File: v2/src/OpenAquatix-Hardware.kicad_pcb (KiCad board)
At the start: 4 copper layers, 96.2 x 96.2 mm, 279 parts, among them J1 USB_B_Micro, J2 Conn_ARM_JTAG_SWD_10, J3 Screw_Terminal_01x02, J4 Screw_Terminal_01x03, Q1 CSD19534Q5A, Q2 BSS138, SW1 SW_Push, SW2 SW_Push, SW3 CJS-1200TA, U1 STM32H723VETx, U10 TPD4E05U06DQA, U11 SSF2215, U12 TPS72301DBV, U13 LM5155DSSR, U14 TLV9061xDBV, U15 OPA333xxD, U16 TLV9061xDBV, U17 PGA113, U18 TPA3132D2RHBR, U19 TLV9151xDBV, U2 TLV75733PDYDR, U20 TLV9151xDBV, U21 SN74LVC1G14DBV, U22 TLP241BTP1_F, U23 TLP241BTP1_F, U24 TLV9061xDBV, U25 TLV9061xDBV, U3 TLV75733PDYDR, U4 TPSM84209RKHR, U5 TPD4E05U06DQA, U6 TPD4E05U06DQA, U7 INA219AIDCNR, U8 SN74LXC1T14DCKR, U9 TPS60403DBV, Y1 8 MHz

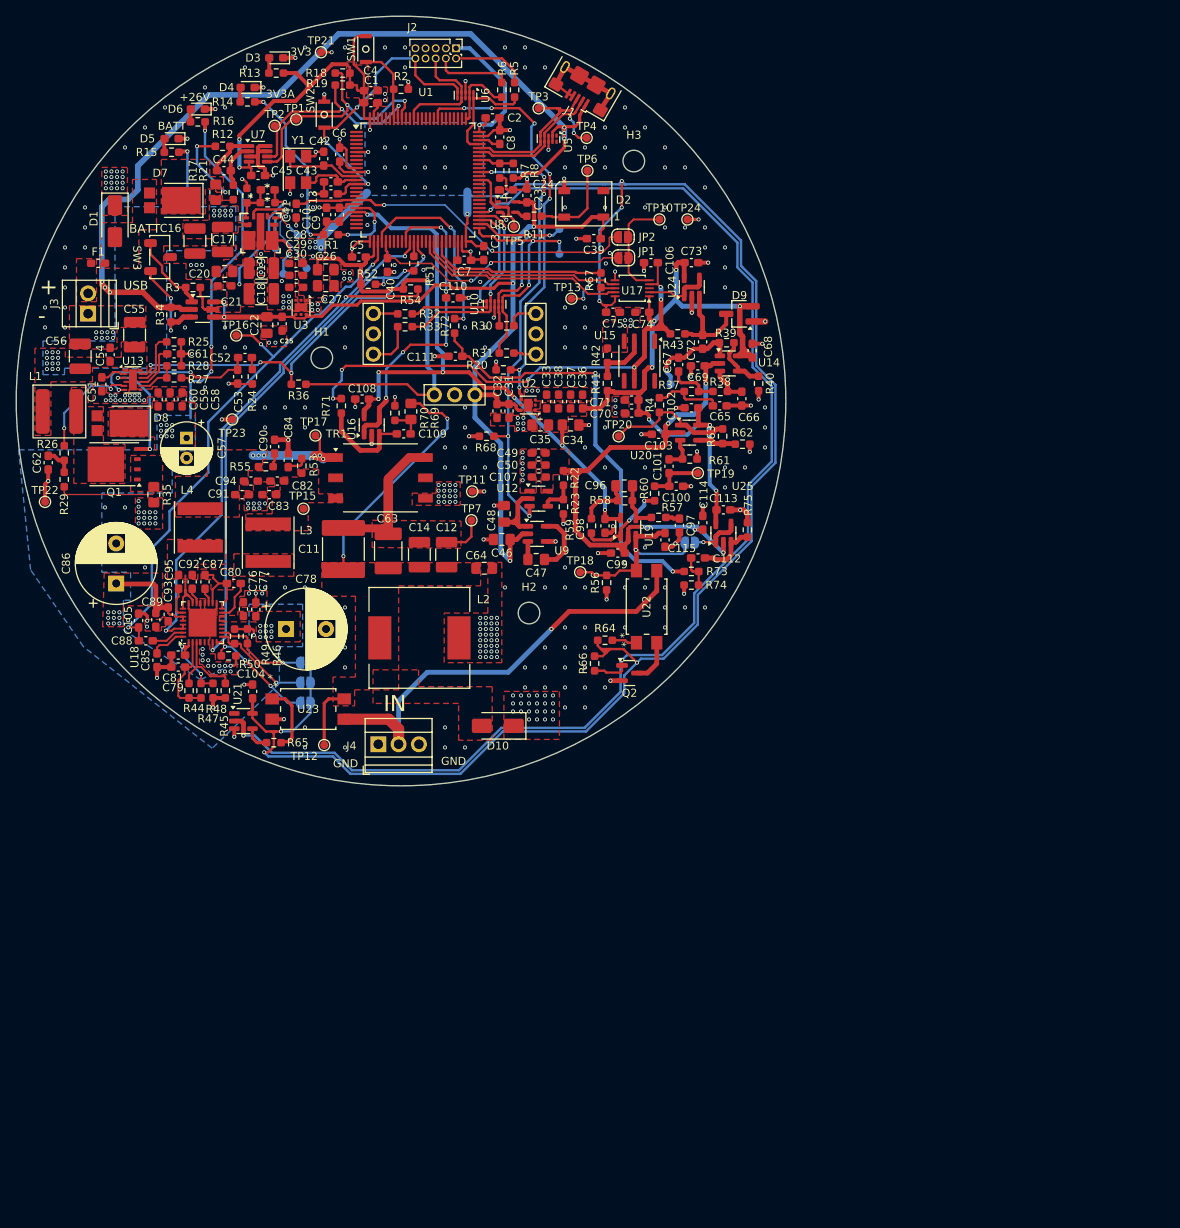
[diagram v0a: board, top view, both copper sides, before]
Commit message: v2.0 final version including minor hardware revisions
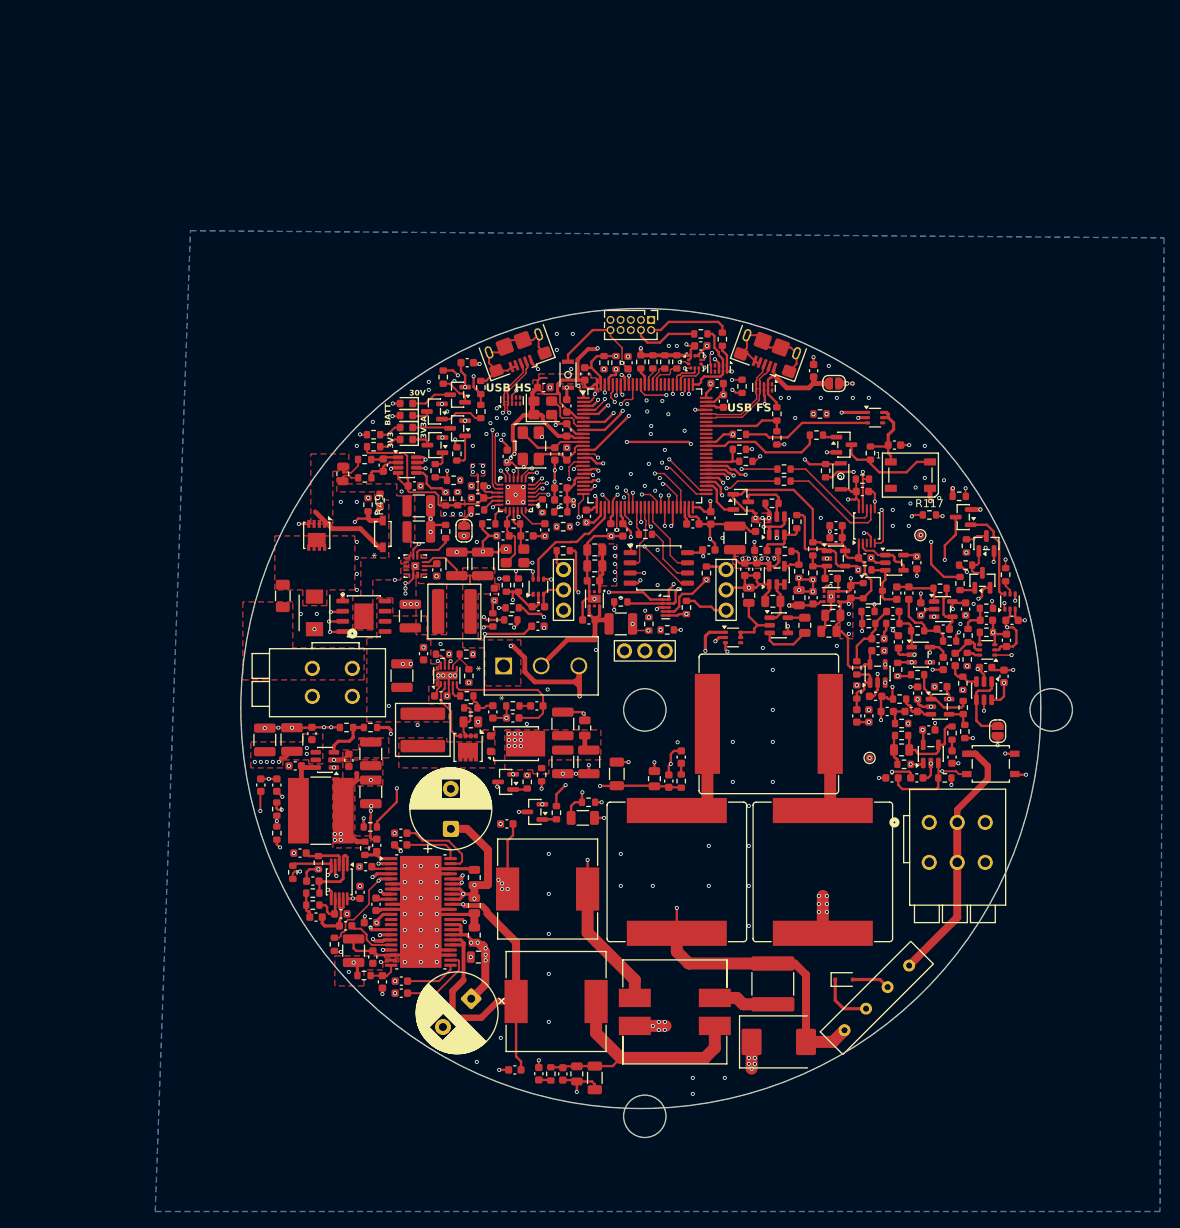
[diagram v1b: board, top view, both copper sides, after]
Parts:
- removed JP4, JP5: SolderJumper_2_Open, Jumper:SolderJumper-2_P1.3mm_Open_RoundedPad1.0x1.5mm
- removed JP6: ~, Jumper:SolderJumper-2_P1.3mm_Open_RoundedPad1.0x1.5mm
- removed TP10, TP14, TP3, TP4, TP5, TP6, TP8, TP9: TestPoint_Small, TestPoint:TestPoint_Pad_D1.0mm
- removed TP11, TP12, TP13, TP15, TP16, TP17, TP18, TP19, TP20, TP21, TP22, TP23, TP24, TP7: TestPoint, TestPoint:TestPoint_Pad_D1.0mm
- removed TP25, TP26, TP27, TP28: ~, TestPoint:TestPoint_Pad_D1.0mm
- removed TR1: Wuerth_760390012, Transformer_SMD:Transformer_Wuerth_750315371
- added C116: 100n, Capacitor_SMD:C_0603_1608Metric, F.Cu at (137.0, 97.1)
- added C117: 100n, Capacitor_SMD:C_0603_1608Metric, F.Cu at (134.1, 97.9)
- added C118: ~, Capacitor_SMD:C_0603_1608Metric, F.Cu at (130.9, 108.5)
- added C119: 33n, Capacitor_SMD:C_0603_1608Metric, F.Cu at (138.4, 105.9)
- added C120: 10u, Capacitor_SMD:C_0805_2012Metric, F.Cu at (132.1, 105.0)
- added C121: 10n, Capacitor_SMD:C_0603_1608Metric, F.Cu at (130.3, 100.2)
- added C122: 2u2, Capacitor_SMD:C_0603_1608Metric, F.Cu at (133.3, 100.2)
- added C123: 68n,200V,5%,C0G/NP0, Capacitor_SMD:C_2220_5750Metric, F.Cu at (116.0, 134.2)
- added C128: 100n, Capacitor_SMD:C_0603_1608Metric, F.Cu at (129.2, 92.6)
- added C129: 100n, Capacitor_SMD:C_0603_1608Metric, F.Cu at (128.8, 98.3)
- added C130: 100n, Capacitor_SMD:C_0603_1608Metric, F.Cu at (137.3, 94.2)
- added C131: 100n, Capacitor_SMD:C_0603_1608Metric, F.Cu at (131.7, 91.5)
- added C132: 1n, Capacitor_SMD:C_0603_1608Metric, F.Cu at (128.0, 100.8)
- added C133: 100n, Capacitor_SMD:C_0603_1608Metric, F.Cu at (140.1, 87.4)
- added C134: 100n, Capacitor_SMD:C_0603_1608Metric, F.Cu at (134.5, 87.4)
- added C135: 1n, Capacitor_SMD:C_0603_1608Metric, F.Cu at (126.5, 100.8)
- added C136: 1n, Capacitor_SMD:C_0603_1608Metric, F.Cu at (129.2, 91.1)
- added C137: 1n, Capacitor_SMD:C_0603_1608Metric, F.Cu at (131.0, 87.7)
- added C138: 1n, Capacitor_SMD:C_0603_1608Metric, F.Cu at (137.3, 89.9)
- added C139: 1n, Capacitor_SMD:C_0603_1608Metric, F.Cu at (133.0, 85.4)
- added C140: 100n, Capacitor_SMD:C_0603_1608Metric, F.Cu at (123.3, 83.6)
- added C141: 100n, Capacitor_SMD:C_0603_1608Metric, F.Cu at (123.9, 78.5)
- added C142: 1u, Capacitor_SMD:C_0603_1608Metric, F.Cu at (123.9, 77.0)
- added C143: 100n, Capacitor_SMD:C_0603_1608Metric, F.Cu at (131.5, 85.4)
- added C144: 100n, Capacitor_SMD:C_0603_1608Metric, F.Cu at (134.0, 81.6)
- added C145: 100n, Capacitor_SMD:C_0603_1608Metric, F.Cu at (127.5, 81.0)
- added C146: 100n, Capacitor_SMD:C_0603_1608Metric, F.Cu at (127.2, 72.7)
- added C147: 100n, Capacitor_SMD:C_0603_1608Metric, F.Cu at (145.9, 88.8)
- added D11: BAT54WS, Diode_SMD:D_SOD-323F, F.Cu at (124.9, 133.7)
- added G***: LOGO, OpenAquatix-Hardware_footprints:OpenAquatix_logo, B.Cu at (100.0, 90.0)
- added J6: 2601-1103, OpenAquatix-Hardware_footprints:CONN3_2601-1103_WAG, F.Cu at (135.6, 114.1)
- added K1: 3570.1419.051, OpenAquatix-Hardware_footprints:3570.1419.xxx, F.Cu at (129.0, 136.0)
- added L5: 33u, OpenAquatix-Hardware_footprints:CDRH127L125NP, F.Cu at (87.8, 122.4)
- added L6: 136u, OpenAquatix-Hardware_footprints:B82477D4xxxM900, F.Cu at (103.8, 137.8)
- added L7: 100u, Inductor_SMD:L_Pulse_PA4344, F.Cu at (104.0, 120.2)
- added L8: 100u, Inductor_SMD:L_Pulse_PA4344, F.Cu at (115.5, 101.8)
- added L9: 100u, Inductor_SMD:L_Pulse_PA4344, F.Cu at (122.2, 120.2)
- added Q10: BSS138, Package_TO_SOT_SMD:SOT-23, F.Cu at (112.0, 74.0)
- added Q11: DMP3068L-7, Package_TO_SOT_SMD:SOT-23, F.Cu at (142.7, 79.2)
- added Q12: BSS138, Package_TO_SOT_SMD:SOT-23, F.Cu at (142.2, 83.8)
- added Q13: BSS138, Package_TO_SOT_SMD:SOT-23, F.Cu at (139.8, 75.9)
- added Q3: Si7617DN, Package_SO:Vishay_PowerPAK_1212-8_Single, F.Cu at (59.0, 78.2)
- added Q4: BSS138, Package_TO_SOT_SMD:SOT-23, F.Cu at (82.6, 109.0)
- added Q5: BSS138, Package_TO_SOT_SMD:SOT-23, F.Cu at (86.2, 112.8)
- added Q6: BSS138, Package_TO_SOT_SMD:SOT-23, F.Cu at (73.8, 66.9)
- added Q7: BSS138, Package_TO_SOT_SMD:SOT-23, F.Cu at (76.6, 64.8)
- added Q8: BSS138, Package_TO_SOT_SMD:SOT-23, F.Cu at (73.7, 62.7)
- added Q9: BSS138, Package_TO_SOT_SMD:SOT-23, F.Cu at (76.6, 60.6)
- added R100: 56k, Resistor_SMD:R_0603_1608Metric, F.Cu at (139.8, 99.7)
- added R101: 8k66, Resistor_SMD:R_0603_1608Metric, F.Cu at (134.1, 95.6)
- added R102: 2k05, Resistor_SMD:R_0603_1608Metric, F.Cu at (131.6, 95.0)
- added R103: 16k9, Resistor_SMD:R_0603_1608Metric, F.Cu at (126.5, 97.8)
- added R104: 10k, Resistor_SMD:R_0603_1608Metric, F.Cu at (126.5, 94.8)
- added R105: 1k91, Resistor_SMD:R_0603_1608Metric, F.Cu at (128.0, 89.2)
- added R106: 28k, Resistor_SMD:R_0603_1608Metric, F.Cu at (131.0, 89.2)
- added R107: 6k19, Resistor_SMD:R_0603_1608Metric, F.Cu at (134.1, 90.1)
- added R108: 1k18, Resistor_SMD:R_0603_1608Metric, F.Cu at (138.1, 91.4)
- added R109: 17k4, Resistor_SMD:R_0603_1608Metric, F.Cu at (136.9, 84.8)
- added R110: 10k, Resistor_SMD:R_0603_1608Metric, F.Cu at (121.0, 79.9)
- added R111: 10k, Resistor_SMD:R_0603_1608Metric, F.Cu at (121.0, 82.9)
- added R112: 10k, Resistor_SMD:R_0603_1608Metric, F.Cu at (127.5, 82.5)
- added R113: 100k, Resistor_SMD:R_0603_1608Metric, F.Cu at (139.3, 73.3)
- added R114: 390R, Resistor_SMD:R_0603_1608Metric, F.Cu at (145.1, 83.1)
- added R115: 100k, Resistor_SMD:R_0603_1608Metric, F.Cu at (127.2, 71.2)
- added R116: 100k, Resistor_SMD:R_0603_1608Metric, F.Cu at (112.2, 59.5)
- added R117: 10k, Resistor_SMD:R_0603_1608Metric, F.Cu at (135.6, 75.6)
- added R76: 100k, Resistor_SMD:R_0603_1608Metric, F.Cu at (79.5, 59.7)
- added R77: 47k, Resistor_SMD:R_0603_1608Metric, F.Cu at (66.9, 73.8)
- added R78: 220R, Resistor_SMD:R_0603_1608Metric, F.Cu at (74.8, 58.4)
- added R79: 100k, Resistor_SMD:R_0603_1608Metric, F.Cu at (96.4, 56.6)
- added R80: 47k, Resistor_SMD:R_0603_1608Metric, F.Cu at (87.1, 108.1)
- added R81: 160k,1%, Resistor_SMD:R_1206_3216Metric, F.Cu at (92.2, 113.5)
- added R82: 1k6,1%, Resistor_SMD:R_0603_1608Metric, F.Cu at (93.0, 111.5)
- added R83: 100k, Resistor_SMD:R_0603_1608Metric, F.Cu at (119.0, 76.5)
- added R84: 2k, Resistor_SMD:R_0603_1608Metric, F.Cu at (115.9, 74.2)
- added R85: 2k49, Resistor_SMD:R_0603_1608Metric, F.Cu at (142.7, 87.3)
- added R86: 732R, Resistor_SMD:R_0603_1608Metric, F.Cu at (140.3, 93.7)
- added R87: 1M, Resistor_SMD:R_0603_1608Metric, F.Cu at (140.4, 90.7)
- added R88: 22R, Resistor_SMD:R_0603_1608Metric, F.Cu at (142.7, 90.3)
- added R89: 100k, Resistor_SMD:R_0603_1608Metric, F.Cu at (139.8, 96.7)
- added R90: 1k, Resistor_SMD:R_0603_1608Metric, F.Cu at (140.2, 79.5)
- added R91: 1k, Resistor_SMD:R_0603_1608Metric, F.Cu at (139.4, 84.2)
- added R92: 100k, Resistor_SMD:R_0603_1608Metric, F.Cu at (140.1, 81.9)
- added R93: 1k, Resistor_SMD:R_0603_1608Metric, F.Cu at (137.5, 108.5)
- added R94: 200R, Resistor_SMD:R_0603_1608Metric, F.Cu at (138.4, 102.9)
- added R95: 91k, Resistor_SMD:R_0603_1608Metric, F.Cu at (132.1, 103.2)
- added R96: 10k, Resistor_SMD:R_0603_1608Metric, F.Cu at (132.4, 106.8)
- added R97: 390R, Resistor_SMD:R_0603_1608Metric, F.Cu at (132.1, 101.7)
- added R98: 86k6, Resistor_SMD:R_0603_1608Metric, F.Cu at (131.8, 98.7)
- added R99: 1k, Resistor_SMD:R_0603_1608Metric, F.Cu at (140.0, 102.7)
- added U26: LM6211, Package_TO_SOT_SMD:SOT-23-5, F.Cu at (135.8, 105.5)
- added U27: LMV641MFX/NOPB, Package_TO_SOT_SMD:SOT-23-5, F.Cu at (136.9, 99.6)
- added U28: LMV641MFX/NOPB, Package_TO_SOT_SMD:SOT-23-5, F.Cu at (129.1, 95.5)
- added U29: LMV641MFX/NOPB, Package_TO_SOT_SMD:SOT-23-5, F.Cu at (134.5, 93.1)
- added U30: LMV641MFX/NOPB, Package_TO_SOT_SMD:SOT-23-5, F.Cu at (137.3, 87.4)
- added U31: LMV641MFX/NOPB, Package_TO_SOT_SMD:SOT-23-5, F.Cu at (123.9, 81.1)
- added U32: LMV641MFX/NOPB, Package_TO_SOT_SMD:SOT-23-5, F.Cu at (131.2, 81.6)
- added U33: PGA113, Package_SO:TSSOP-10_3x3mm_P0.5mm, F.Cu at (127.8, 77.0)
- added U34: TS5A4624, Package_TO_SOT_SMD:SOT-363_SC-70-6, F.Cu at (145.7, 86.5)
- added U35: AQY210S, OpenAquatix-Hardware_footprints:RELAY_AQY_SO4_KS_PAN, F.Cu at (143.2, 106.8)
- added Y2: 8 MHz, Crystal:Crystal_SMD_5032-4Pin_5.0x3.2mm, F.Cu at (85.8, 67.0)
- added Y3: 26 MHz, Crystal:Crystal_SMD_3225-4Pin_3.2x2.5mm, F.Cu at (83.8, 80.8)
- C1, C104, C108, C112, C113, C114, C29, C6, C61, C68, C71, C81, C85, C9: footprint Capacitor_SMD:C_0603_1608Metric_Pad1.08x0.95mm_HandSolder -> Capacitor_SMD:C_0603_1608Metric
- C10, C79: value 1u -> 100n; footprint Capacitor_SMD:C_0603_1608Metric_Pad1.08x0.95mm_HandSolder -> Capacitor_SMD:C_0603_1608Metric
- C100: value 10n -> 1n,50V; footprint Capacitor_SMD:C_0603_1608Metric_Pad1.08x0.95mm_HandSolder -> Capacitor_SMD:C_0603_1608Metric
- C101: value 2u2 -> 1n,50V; footprint Capacitor_SMD:C_0603_1608Metric_Pad1.08x0.95mm_HandSolder -> Capacitor_SMD:C_0603_1608Metric
- C102, C103: value 100n -> 10n,50V; footprint Capacitor_SMD:C_0603_1608Metric_Pad1.08x0.95mm_HandSolder -> Capacitor_SMD:C_0603_1608Metric
- C105: value 1n -> 1u; footprint Capacitor_SMD:C_0603_1608Metric_Pad1.08x0.95mm_HandSolder -> Capacitor_SMD:C_0603_1608Metric
- C106, C65: value C -> 100n; footprint Capacitor_SMD:C_0603_1608Metric_Pad1.08x0.95mm_HandSolder -> Capacitor_SMD:C_0603_1608Metric
- C107, C38: value 1n -> 100n; footprint Capacitor_SMD:C_0603_1608Metric_Pad1.08x0.95mm_HandSolder -> Capacitor_SMD:C_0603_1608Metric
- C109, C69: value 100n -> 1n; footprint Capacitor_SMD:C_0603_1608Metric_Pad1.08x0.95mm_HandSolder -> Capacitor_SMD:C_0603_1608Metric
- C11: value C -> 100n; footprint Capacitor_SMD:C_2220_5750Metric_Pad1.97x5.40mm_HandSolder -> Capacitor_SMD:C_0603_1608Metric
- C110, C40, C41: value 47p -> 100n; footprint Capacitor_SMD:C_0603_1608Metric_Pad1.08x0.95mm_HandSolder -> Capacitor_SMD:C_0603_1608Metric
- C111: value 1n -> 10u; footprint Capacitor_SMD:C_0603_1608Metric_Pad1.08x0.95mm_HandSolder -> Capacitor_SMD:C_0603_1608Metric
- C115: value ~ -> 100n; footprint Capacitor_SMD:C_0603_1608Metric_Pad1.08x0.95mm_HandSolder -> Capacitor_SMD:C_0603_1608Metric
- C12: value C -> 8p; footprint Capacitor_SMD:C_1210_3225Metric_Pad1.33x2.70mm_HandSolder -> Capacitor_SMD:C_0603_1608Metric
- C13: value 100n -> 47p; footprint Capacitor_SMD:C_0603_1608Metric_Pad1.08x0.95mm_HandSolder -> Capacitor_SMD:C_0603_1608Metric
- C14: value C -> 100n; footprint Capacitor_SMD:C_1210_3225Metric_Pad1.33x2.70mm_HandSolder -> Capacitor_SMD:C_0603_1608Metric
- C15: value 330p -> 4u7; footprint Capacitor_SMD:C_0603_1608Metric_Pad1.08x0.95mm_HandSolder -> Capacitor_SMD:C_0603_1608Metric
- C16: value 10u,50V -> 47p; footprint Capacitor_SMD:C_1210_3225Metric_Pad1.33x2.70mm_HandSolder -> Capacitor_SMD:C_0603_1608Metric
- C17: value 10u,50V -> 8p; footprint Capacitor_SMD:C_1210_3225Metric_Pad1.33x2.70mm_HandSolder -> Capacitor_SMD:C_0603_1608Metric
- C18, C19: value 47u -> 100n; footprint Capacitor_SMD:C_1210_3225Metric_Pad1.33x2.70mm_HandSolder -> Capacitor_SMD:C_0603_1608Metric
- C2, C24: value 100n -> 1u; footprint Capacitor_SMD:C_0603_1608Metric_Pad1.08x0.95mm_HandSolder -> Capacitor_SMD:C_0603_1608Metric
- C20: value 10u -> 1u; footprint Capacitor_SMD:C_0805_2012Metric_Pad1.18x1.45mm_HandSolder -> Capacitor_SMD:C_0603_1608Metric
- C21: value 1u -> 10u,50V; footprint Capacitor_SMD:C_0603_1608Metric_Pad1.08x0.95mm_HandSolder -> Capacitor_SMD:C_1210_3225Metric
- C22, C26: value 22u -> 10u,50V; footprint Capacitor_SMD:C_0805_2012Metric_Pad1.18x1.45mm_HandSolder -> Capacitor_SMD:C_1210_3225Metric
- C23: value 100n -> 330n; footprint Capacitor_SMD:C_0603_1608Metric_Pad1.08x0.95mm_HandSolder -> Capacitor_SMD:C_0603_1608Metric
- C25, C31: value 100n -> 2u2; footprint Capacitor_SMD:C_0603_1608Metric_Pad1.08x0.95mm_HandSolder -> Capacitor_SMD:C_0805_2012Metric
- C27: value 22u -> 4u7,50V; footprint Capacitor_SMD:C_0805_2012Metric_Pad1.18x1.45mm_HandSolder -> Capacitor_SMD:C_1210_3225Metric
- C28: value 1u -> 68p; footprint Capacitor_SMD:C_0603_1608Metric_Pad1.08x0.95mm_HandSolder -> Capacitor_SMD:C_0603_1608Metric
- C3, C5: value 100n -> 2u2; footprint Capacitor_SMD:C_0603_1608Metric_Pad1.08x0.95mm_HandSolder -> Capacitor_SMD:C_0603_1608Metric
- C30: value 1n -> 10n; footprint Capacitor_SMD:C_0603_1608Metric_Pad1.08x0.95mm_HandSolder -> Capacitor_SMD:C_0603_1608Metric
- C32: value 10u -> 2u2; footprint Capacitor_SMD:C_0603_1608Metric_Pad1.08x0.95mm_HandSolder -> Capacitor_SMD:C_0805_2012Metric
- C33: value 100p -> 1u; footprint Capacitor_SMD:C_0603_1608Metric_Pad1.08x0.95mm_HandSolder -> Capacitor_SMD:C_0603_1608Metric
- C34: value 22u -> 47u; footprint Capacitor_SMD:C_0805_2012Metric_Pad1.18x1.45mm_HandSolder -> Capacitor_SMD:C_1210_3225Metric
- C35: footprint Capacitor_SMD:C_0805_2012Metric_Pad1.18x1.45mm_HandSolder -> Capacitor_SMD:C_1210_3225Metric
- C36: value 1u -> 1n; footprint Capacitor_SMD:C_0603_1608Metric_Pad1.08x0.95mm_HandSolder -> Capacitor_SMD:C_0603_1608Metric
- C37: value 100n -> 22u; footprint Capacitor_SMD:C_0603_1608Metric_Pad1.08x0.95mm_HandSolder -> Capacitor_SMD:C_1210_3225Metric
- C39: value 100n -> 4u7; footprint Capacitor_SMD:C_0603_1608Metric_Pad1.08x0.95mm_HandSolder -> Capacitor_SMD:C_0603_1608Metric
- C4: value 4u7 -> 100n; footprint Capacitor_SMD:C_0603_1608Metric_Pad1.08x0.95mm_HandSolder -> Capacitor_SMD:C_0603_1608Metric
- C42: value 8p -> 100n; footprint Capacitor_SMD:C_0603_1608Metric_Pad1.08x0.95mm_HandSolder -> Capacitor_SMD:C_0603_1608Metric
- C43: value 8p -> 10u; footprint Capacitor_SMD:C_0603_1608Metric_Pad1.08x0.95mm_HandSolder -> Capacitor_SMD:C_0805_2012Metric
- C44: value 1u -> 22u; footprint Capacitor_SMD:C_0603_1608Metric_Pad1.08x0.95mm_HandSolder -> Capacitor_SMD:C_1210_3225Metric
- C45: value 100n -> 10u,63V; footprint Capacitor_SMD:C_0603_1608Metric_Pad1.08x0.95mm_HandSolder -> Capacitor_SMD:C_1210_3225Metric
- C46, C47: value 2u2 -> 10u,63V; footprint Capacitor_SMD:C_0805_2012Metric_Pad1.18x1.45mm_HandSolder -> Capacitor_SMD:C_1210_3225Metric
- C48: value 2u2 -> 22u; footprint Capacitor_SMD:C_0805_2012Metric_Pad1.18x1.45mm_HandSolder -> Capacitor_SMD:C_0805_2012Metric
- C49: value 4u7 -> 1u,100V; footprint Capacitor_SMD:C_0603_1608Metric_Pad1.08x0.95mm_HandSolder -> Capacitor_SMD:C_0805_2012Metric
- C50: value 100n -> 22u; footprint Capacitor_SMD:C_0603_1608Metric_Pad1.08x0.95mm_HandSolder -> Capacitor_SMD:C_0805_2012Metric
- C51: value 1u -> 22u; footprint Capacitor_SMD:C_0603_1608Metric_Pad1.08x0.95mm_HandSolder -> Capacitor_SMD:C_0805_2012Metric
- C52: value 27n -> 22u; footprint Capacitor_SMD:C_0603_1608Metric_Pad1.08x0.95mm_HandSolder -> Capacitor_SMD:C_0805_2012Metric
- C53: value 22n -> 100n; footprint Capacitor_SMD:C_0603_1608Metric_Pad1.08x0.95mm_HandSolder -> Capacitor_SMD:C_0603_1608Metric
- C54, C77: value 100n,50V -> 100n; footprint Capacitor_SMD:C_0603_1608Metric_Pad1.08x0.95mm_HandSolder -> Capacitor_SMD:C_0603_1608Metric
- C55, C56: value 10u,50V -> 4u7,50V; footprint Capacitor_SMD:C_1210_3225Metric_Pad1.33x2.70mm_HandSolder -> Capacitor_SMD:C_1210_3225Metric
- C57: value 68u -> 100n; footprint Capacitor_THT:CP_Radial_D6.3mm_P2.50mm -> Capacitor_SMD:C_0603_1608Metric
- C58: value 1u,50V -> 100n; footprint Capacitor_SMD:C_0603_1608Metric_Pad1.08x0.95mm_HandSolder -> Capacitor_SMD:C_0603_1608Metric
- C59: value 1u,50V -> 22u,25V; footprint Capacitor_SMD:C_0603_1608Metric_Pad1.08x0.95mm_HandSolder -> Capacitor_SMD:C_1210_3225Metric
- C60: value 100n,50V -> 22u,25V; footprint Capacitor_SMD:C_0603_1608Metric_Pad1.08x0.95mm_HandSolder -> Capacitor_SMD:C_1210_3225Metric
- C62: value 1n -> 30p; footprint Capacitor_SMD:C_0603_1608Metric_Pad1.08x0.95mm_HandSolder -> Capacitor_SMD:C_0603_1608Metric
- C63: value 68n,200V,5%,C0G/NP0 -> 1u; footprint Capacitor_SMD:C_1812_4532Metric_Pad1.57x3.40mm_HandSolder -> Capacitor_SMD:C_0603_1608Metric
- C64: value C -> 30p; footprint Capacitor_SMD:C_0805_2012Metric_Pad1.18x1.45mm_HandSolder -> Capacitor_SMD:C_0603_1608Metric
- C66: value 100p -> 2u2; footprint Capacitor_SMD:C_0603_1608Metric_Pad1.08x0.95mm_HandSolder -> Capacitor_SMD:C_0603_1608Metric
- C67: value 240p -> 2u2; footprint Capacitor_SMD:C_0603_1608Metric_Pad1.08x0.95mm_HandSolder -> Capacitor_SMD:C_0603_1608Metric
- C7, C8: value 2u2 -> 100n; footprint Capacitor_SMD:C_0603_1608Metric_Pad1.08x0.95mm_HandSolder -> Capacitor_SMD:C_0603_1608Metric
- C70: value 1u -> 1n2; footprint Capacitor_SMD:C_0603_1608Metric_Pad1.08x0.95mm_HandSolder -> Capacitor_SMD:C_0603_1608Metric
- C72: value 100n -> 100p; footprint Capacitor_SMD:C_0603_1608Metric_Pad1.08x0.95mm_HandSolder -> Capacitor_SMD:C_0603_1608Metric
- C73: value 100n -> 6n8; footprint Capacitor_SMD:C_0603_1608Metric_Pad1.08x0.95mm_HandSolder -> Capacitor_SMD:C_0603_1608Metric
- C74: value 100n -> 1u; footprint Capacitor_SMD:C_0603_1608Metric_Pad1.08x0.95mm_HandSolder -> Capacitor_SMD:C_0805_2012Metric
- C75: value 100n -> 10u; footprint Capacitor_SMD:C_0603_1608Metric_Pad1.08x0.95mm_HandSolder -> Capacitor_SMD:C_1210_3225Metric
- C76, C82: value 1n,50V -> 1u; footprint Capacitor_SMD:C_0603_1608Metric_Pad1.08x0.95mm_HandSolder -> Capacitor_SMD:C_0805_2012Metric
- C78: value 220u -> 470u
- C80: value 220n,50V -> 100n; footprint Capacitor_SMD:C_0603_1608Metric_Pad1.08x0.95mm_HandSolder -> Capacitor_SMD:C_0603_1608Metric
- C83: value 220n,100V -> 10n; footprint Capacitor_SMD:C_0603_1608Metric_Pad1.08x0.95mm_HandSolder -> Capacitor_SMD:C_0603_1608Metric
- C84: value 10n,50V -> 1u; footprint Capacitor_SMD:C_0603_1608Metric_Pad1.08x0.95mm_HandSolder -> Capacitor_SMD:C_0805_2012Metric
- C86: value 220u -> 1u; footprint Capacitor_THT:CP_Radial_D10.0mm_P5.00mm -> Capacitor_SMD:C_0603_1608Metric
- C87: value 220n,50V -> 1u; footprint Capacitor_SMD:C_0603_1608Metric_Pad1.08x0.95mm_HandSolder -> Capacitor_SMD:C_0603_1608Metric
- C88: value 1u -> 470u; footprint Capacitor_SMD:C_0603_1608Metric_Pad1.08x0.95mm_HandSolder -> Capacitor_THT:CP_Radial_D10.0mm_P5.00mm
- C89: value 100n,50V -> 33n; footprint Capacitor_SMD:C_0603_1608Metric_Pad1.08x0.95mm_HandSolder -> Capacitor_SMD:C_0603_1608Metric
- C90: value 10n,50V -> 33n; footprint Capacitor_SMD:C_0603_1608Metric_Pad1.08x0.95mm_HandSolder -> Capacitor_SMD:C_0603_1608Metric
- C91: value 220n,100V -> 100n; footprint Capacitor_SMD:C_0603_1608Metric_Pad1.08x0.95mm_HandSolder -> Capacitor_SMD:C_0603_1608Metric
- C92: value 220n,50V -> 33n; footprint Capacitor_SMD:C_0603_1608Metric_Pad1.08x0.95mm_HandSolder -> Capacitor_SMD:C_0603_1608Metric
- C93: value 1n,50V -> 33n; footprint Capacitor_SMD:C_0603_1608Metric_Pad1.08x0.95mm_HandSolder -> Capacitor_SMD:C_0603_1608Metric
- C94: value 1n,50V -> 1n; footprint Capacitor_SMD:C_0603_1608Metric_Pad1.08x0.95mm_HandSolder -> Capacitor_SMD:C_0603_1608Metric
- C95: value 220n,50V -> 1n; footprint Capacitor_SMD:C_0603_1608Metric_Pad1.08x0.95mm_HandSolder -> Capacitor_SMD:C_0603_1608Metric
- C96: value 10u -> 680n,100V; footprint Capacitor_SMD:C_0805_2012Metric_Pad1.18x1.45mm_HandSolder -> Capacitor_SMD:C_1206_3216Metric
- C97: value 33n -> 680n,100V; footprint Capacitor_SMD:C_0603_1608Metric_Pad1.08x0.95mm_HandSolder -> Capacitor_SMD:C_1206_3216Metric
- C98, C99: value 100n -> 220n,100V; footprint Capacitor_SMD:C_0603_1608Metric_Pad1.08x0.95mm_HandSolder -> Capacitor_SMD:C_0805_2012Metric
- D1: value SMBJ24CA -> WS2812B; footprint Diode_SMD:D_SMA -> LED_SMD:LED_WS2812B_PLCC4_5.0x5.0mm_P3.2mm
- D10: value 5.0SMDJ78CA -> 1SS396,LF; footprint Diode_SMD:D_SMA -> Package_TO_SOT_SMD:SC-59
- D2: value WS2812B -> PDS760-13; footprint LED_SMD:LED_WS2812B_PLCC4_5.0x5.0mm_P3.2mm -> Package_TO_SOT_SMD:TO-277B
- D3: value Red -> SMBJ24CA; footprint LED_SMD:LED_0603_1608Metric_Pad1.05x0.95mm_HandSolder -> OpenAquatix-Hardware_footprints:SMBJ
- D4: value Red -> MMSZ12T1G; footprint LED_SMD:LED_0603_1608Metric_Pad1.05x0.95mm_HandSolder -> OpenAquatix-Hardware_footprints:SOD-123_ONS
- D5, D6: footprint LED_SMD:LED_0603_1608Metric_Pad1.05x0.95mm_HandSolder -> Diode_SMD:D_0603_1608Metric
- D7, D8: value SDT10A45P5-7 -> Red; footprint Diodes:PowerDI-5 -> Diode_SMD:D_0603_1608Metric
- D9: value 1SS396,LF -> SMLJ150CA; footprint Package_TO_SOT_SMD:SC-59_Handsoldering -> Diode_SMD:D_SMC
- F1: value 5A -> 6A; footprint Fuse:Fuse_0603_1608Metric_Pad1.05x0.95mm_HandSolder -> Fuse:Fuse_1206_3216Metric
- H1, H2, H3: footprint MountingHole:MountingHole_2.7mm_M2.5_ISO14580 -> MountingHole:MountingHole_5.3mm_M5
- J1: value USB_B_Micro -> Conn_ARM_JTAG_SWD_10; footprint Connector_USB:USB_Micro-B_Amphenol_10118193-0001LF_Horizontal -> Connector_PinHeader_1.27mm:PinHeader_2x05_P1.27mm_Vertical
- J2: value Conn_ARM_JTAG_SWD_10 -> USB_B_Micro; footprint Connector_PinHeader_1.27mm:PinHeader_2x05_P1.27mm_Vertical -> Connector_USB:USB_Micro-B_Amphenol_10118193-0001LF_Horizontal
- J3: value Screw_Terminal_01x02 -> USB_B_Micro; footprint TerminalBlock:TerminalBlock_Xinya_XY308-2.54-2P_1x02_P2.54mm_Horizontal -> Connector_USB:USB_Micro-B_Amphenol_10118193-0001LF_Horizontal
- J4: value Screw_Terminal_01x03 -> ~; footprint TerminalBlock:TerminalBlock_Xinya_XY308-2.54-3P_1x03_P2.54mm_Horizontal -> OpenAquatix-Hardware_footprints:UAM_DaughterCard
- J5: value ~ -> 2601-1102; footprint Connections:UAM_DaughterCard -> OpenAquatix-Hardware_footprints:CONN2_2601-1102_WAG
- JP1, JP2: value SolderJumper_2_Open -> ~
- JP3: value SolderJumper_2_Open -> ~; moved to F.Cu
- L1: value 4u7 -> 6u8; footprint Inductor:SRP6060FA -> Inductor_SMD:L_Bourns_SRP6060FA
- L2: value 270u -> 15u; footprint Inductor_SMD:L_12x12mm_H8mm -> Inductor_SMD:L_Bourns_SRP6060FA
- L3: value 22u -> 33u; footprint NRS6045T100MMGK:IND_TAIYO_NRS6045_TAY -> Inductor_SMD:L_Bourns-SRN8040_8x8.15mm
- L4: value 22u -> 33u; footprint NRS6045T100MMGK:IND_TAIYO_NRS6045_TAY -> OpenAquatix-Hardware_footprints:CDRH127L125NP
- Q1: value CSD19534Q5A -> BSS138; footprint Package_TO_SOT_SMD:TDSON-8-1 -> Package_TO_SOT_SMD:SOT-23
- Q2: value BSS138 -> CSD18543Q3A; footprint Package_TO_SOT_SMD:SOT-23 -> Package_SON:VSON-8_3.3x3.3mm_P0.65mm_NexFET
- R1: value 47R -> 4k7; footprint Resistor_SMD:R_0603_1608Metric_Pad0.98x0.95mm_HandSolder -> Resistor_SMD:R_0603_1608Metric
- R10: value 1k37 -> 2k49; footprint Resistor_SMD:R_0603_1608Metric_Pad0.98x0.95mm_HandSolder -> Resistor_SMD:R_0603_1608Metric
- R11: value 470R -> 2k49; footprint Resistor_SMD:R_0603_1608Metric_Pad0.98x0.95mm_HandSolder -> Resistor_SMD:R_0603_1608Metric
- R12: value 100R -> 33k; footprint Resistor_SMD:R_0603_1608Metric_Pad0.98x0.95mm_HandSolder -> Resistor_SMD:R_0603_1608Metric
- R13: value 470R -> 56k; footprint Resistor_SMD:R_0603_1608Metric_Pad0.98x0.95mm_HandSolder -> Resistor_SMD:R_0603_1608Metric
- R14: value 470R -> 390R; footprint Resistor_SMD:R_0603_1608Metric_Pad0.98x0.95mm_HandSolder -> Resistor_SMD:R_0603_1608Metric
- R15, R19, R71, R74: value 10k -> 2k; footprint Resistor_SMD:R_0603_1608Metric_Pad0.98x0.95mm_HandSolder -> Resistor_SMD:R_0603_1608Metric
- R16, R9: value 10k -> 22R; footprint Resistor_SMD:R_0603_1608Metric_Pad0.98x0.95mm_HandSolder -> Resistor_SMD:R_0603_1608Metric
- R17: value 10m -> 22R; footprint Resistor_SMD:R_0805_2012Metric_Pad1.20x1.40mm_HandSolder -> Resistor_SMD:R_0603_1608Metric
- R18, R20, R50: value 10k -> 100k; footprint Resistor_SMD:R_0603_1608Metric_Pad0.98x0.95mm_HandSolder -> Resistor_SMD:R_0603_1608Metric
- R2, R3, R43: value 10k -> 4k7; footprint Resistor_SMD:R_0603_1608Metric_Pad0.98x0.95mm_HandSolder -> Resistor_SMD:R_0603_1608Metric
- R21: value 100R -> 2k; footprint Resistor_SMD:R_0603_1608Metric_Pad0.98x0.95mm_HandSolder -> Resistor_SMD:R_0603_1608Metric
- R22: value 82k -> 4k7; footprint Resistor_SMD:R_0603_1608Metric_Pad0.98x0.95mm_HandSolder -> Resistor_SMD:R_0603_1608Metric
- R23: value 20k -> 4k7; footprint Resistor_SMD:R_0603_1608Metric_Pad0.98x0.95mm_HandSolder -> Resistor_SMD:R_0603_1608Metric
- R24: value 3k3 -> 28k7; footprint Resistor_SMD:R_0603_1608Metric_Pad0.98x0.95mm_HandSolder -> Resistor_SMD:R_0603_1608Metric
- R25: value 26k7 -> 1k; footprint Resistor_SMD:R_0603_1608Metric_Pad0.98x0.95mm_HandSolder -> Resistor_SMD:R_0603_1608Metric
- R26: value 383R -> 100k; footprint Resistor_SMD:R_0603_1608Metric_Pad0.98x0.95mm_HandSolder -> Resistor_SMD:R_0603_1608Metric
- R27: value 62k -> 150k; footprint Resistor_SMD:R_0603_1608Metric_Pad0.98x0.95mm_HandSolder -> Resistor_SMD:R_0603_1608Metric
- R28: value 2k49 -> 21k; footprint Resistor_SMD:R_0603_1608Metric_Pad0.98x0.95mm_HandSolder -> Resistor_SMD:R_0603_1608Metric
- R29: value 100R -> 10k; footprint Resistor_SMD:R_0603_1608Metric_Pad0.98x0.95mm_HandSolder -> Resistor_SMD:R_0603_1608Metric
- R30: value 100R -> 267R; footprint Resistor_SMD:R_0603_1608Metric_Pad0.98x0.95mm_HandSolder -> Resistor_SMD:R_0603_1608Metric
- R31: value 100R -> 68k; footprint Resistor_SMD:R_0603_1608Metric_Pad0.98x0.95mm_HandSolder -> Resistor_SMD:R_0603_1608Metric
- R32: value 330R -> 39k; footprint Resistor_SMD:R_0603_1608Metric_Pad0.98x0.95mm_HandSolder -> Resistor_SMD:R_0603_1608Metric
- R33: value 330R -> 100R; footprint Resistor_SMD:R_0603_1608Metric_Pad0.98x0.95mm_HandSolder -> Resistor_SMD:R_0603_1608Metric
- R34, R66: value 10k -> 10m; footprint Resistor_SMD:R_0603_1608Metric_Pad0.98x0.95mm_HandSolder -> Resistor_SMD:R_0805_2012Metric
- R35: value 10m -> 71k5; footprint Resistor_SMD:R_0805_2012Metric_Pad1.20x1.40mm_HandSolder -> Resistor_SMD:R_0603_1608Metric
- R36: value 10k -> 2k49; footprint Resistor_SMD:R_0603_1608Metric_Pad0.98x0.95mm_HandSolder -> Resistor_SMD:R_0603_1608Metric
- R37: value 16k -> 10k; footprint Resistor_SMD:R_0603_1608Metric_Pad0.98x0.95mm_HandSolder -> Resistor_SMD:R_0603_1608Metric
- R38: value 39k -> 300k; footprint Resistor_SMD:R_0603_1608Metric_Pad0.98x0.95mm_HandSolder -> Resistor_SMD:R_0603_1608Metric
- R39: value 0R -> 22k; footprint Resistor_SMD:R_0603_1608Metric_Pad0.98x0.95mm_HandSolder -> Resistor_SMD:R_0603_1608Metric
- R4: value 0R -> 47R; footprint Resistor_SMD:R_0603_1608Metric_Pad0.98x0.95mm_HandSolder -> Resistor_SMD:R_0603_1608Metric
- R40: value ~ -> 390R; footprint Resistor_SMD:R_0603_1608Metric_Pad0.98x0.95mm_HandSolder -> Resistor_SMD:R_0603_1608Metric
- R41, R46: value 10k -> 390R; footprint Resistor_SMD:R_0603_1608Metric_Pad0.98x0.95mm_HandSolder -> Resistor_SMD:R_0603_1608Metric
- R42: value 10k -> 20k; footprint Resistor_SMD:R_0603_1608Metric_Pad0.98x0.95mm_HandSolder -> Resistor_SMD:R_0603_1608Metric
- R44: value 5k6 -> 1M; footprint Resistor_SMD:R_0603_1608Metric_Pad0.98x0.95mm_HandSolder -> Resistor_SMD:R_0603_1608Metric
- R45: value ~ -> 8k06; footprint Resistor_SMD:R_0603_1608Metric_Pad0.98x0.95mm_HandSolder -> Resistor_SMD:R_0603_1608Metric
- R47: value 56k -> 390R; footprint Resistor_SMD:R_0603_1608Metric_Pad0.98x0.95mm_HandSolder -> Resistor_SMD:R_0603_1608Metric
- R48: value 36k -> 22R; footprint Resistor_SMD:R_0603_1608Metric_Pad0.98x0.95mm_HandSolder -> Resistor_SMD:R_0603_1608Metric
- R49: value 10k -> 1M; footprint Resistor_SMD:R_0603_1608Metric_Pad0.98x0.95mm_HandSolder -> Resistor_SMD:R_0603_1608Metric
- R5: value 22R -> 4k7; footprint Resistor_SMD:R_0603_1608Metric_Pad0.98x0.95mm_HandSolder -> Resistor_SMD:R_0603_1608Metric
- R51: value 330R -> 470R; footprint Resistor_SMD:R_0603_1608Metric_Pad0.98x0.95mm_HandSolder -> Resistor_SMD:R_0603_1608Metric
- R52: value 10k -> 499R; footprint Resistor_SMD:R_0603_1608Metric_Pad0.98x0.95mm_HandSolder -> Resistor_SMD:R_0603_1608Metric
- R53: value 3R3 -> 100k; footprint Resistor_SMD:R_0603_1608Metric_Pad0.98x0.95mm_HandSolder -> Resistor_SMD:R_0603_1608Metric
- R54: value 10k -> 470R; footprint Resistor_SMD:R_0603_1608Metric_Pad0.98x0.95mm_HandSolder -> Resistor_SMD:R_0603_1608Metric
- R55: value 3R3 -> 2k94; footprint Resistor_SMD:R_0603_1608Metric_Pad0.98x0.95mm_HandSolder -> Resistor_SMD:R_0603_1608Metric
- R56: value 100k -> 10k; footprint Resistor_SMD:R_0603_1608Metric_Pad0.98x0.95mm_HandSolder -> Resistor_SMD:R_0603_1608Metric
- R57: value 200R -> 10k; footprint Resistor_SMD:R_0603_1608Metric_Pad0.98x0.95mm_HandSolder -> Resistor_SMD:R_0603_1608Metric
- R58: value 91k -> 806R; footprint Resistor_SMD:R_0603_1608Metric_Pad0.98x0.95mm_HandSolder -> Resistor_SMD:R_0603_1608Metric
- R59: value 10k -> 1k21; footprint Resistor_SMD:R_0603_1608Metric_Pad0.98x0.95mm_HandSolder -> Resistor_SMD:R_0603_1608Metric
- R6: value 22R -> 10k; footprint Resistor_SMD:R_0603_1608Metric_Pad0.98x0.95mm_HandSolder -> Resistor_SMD:R_0603_1608Metric
- R60: value 392R -> 3R3; footprint Resistor_SMD:R_0603_1608Metric_Pad0.98x0.95mm_HandSolder -> Resistor_SMD:R_0603_1608Metric
- R61: value 86k6 -> 3R3; footprint Resistor_SMD:R_0603_1608Metric_Pad0.98x0.95mm_HandSolder -> Resistor_SMD:R_0603_1608Metric
- R62: value 1k -> 22k; footprint Resistor_SMD:R_0603_1608Metric_Pad0.98x0.95mm_HandSolder -> Resistor_SMD:R_0603_1608Metric
- R63: value 56k -> 30k,1%; footprint Resistor_SMD:R_0603_1608Metric_Pad0.98x0.95mm_HandSolder -> Resistor_SMD:R_0603_1608Metric
- R64, R65: value 150R -> 3R3; footprint Resistor_SMD:R_0603_1608Metric_Pad0.98x0.95mm_HandSolder -> Resistor_SMD:R_0603_1608Metric
- R67: value 1k -> 100R; footprint Resistor_SMD:R_0603_1608Metric_Pad0.98x0.95mm_HandSolder -> Resistor_SMD:R_0603_1608Metric
- R68: value 10k -> 100R; footprint Resistor_SMD:R_0603_1608Metric_Pad0.98x0.95mm_HandSolder -> Resistor_SMD:R_0603_1608Metric
- R69: value 160k,1% -> 220R; footprint Resistor_SMD:R_0805_2012Metric_Pad1.20x1.40mm_HandSolder -> Resistor_SMD:R_0603_1608Metric
- R7: value 56k -> 22R; footprint Resistor_SMD:R_0603_1608Metric_Pad0.98x0.95mm_HandSolder -> Resistor_SMD:R_0603_1608Metric
- R70: value 2k,1% -> 100k; footprint Resistor_SMD:R_0603_1608Metric_Pad0.98x0.95mm_HandSolder -> Resistor_SMD:R_0603_1608Metric
- R72: value 2k49 -> 220R; footprint Resistor_SMD:R_0603_1608Metric_Pad0.98x0.95mm_HandSolder -> Resistor_SMD:R_0603_1608Metric
- R73: value 1M -> 100k; footprint Resistor_SMD:R_0603_1608Metric_Pad0.98x0.95mm_HandSolder -> Resistor_SMD:R_0603_1608Metric
- R75: value 10k -> 220R; footprint Resistor_SMD:R_0603_1608Metric_Pad0.98x0.95mm_HandSolder -> Resistor_SMD:R_0603_1608Metric
- R8: value 33k -> 1k; footprint Resistor_SMD:R_0603_1608Metric_Pad0.98x0.95mm_HandSolder -> Resistor_SMD:R_0603_1608Metric
- SW1, SW2: footprint Switches:EVP-AWED4A (3.00mm x 2.00mm) -> OpenAquatix-Hardware_footprints:EVP-AWED4A (3.00mm x 2.00mm)
- SW3: value CJS-1200TA -> CS12ANW03; footprint Switches:CJS-1200TA -> OpenAquatix-Hardware_footprints:CS12ANW03_NKK
- TP1, TP2: value TestPoint_Small -> TestPoint
- U1: value STM32H723VETx -> W25Q16JVSS; footprint Package_QFP:LQFP-100_14x14mm_P0.5mm -> Package_SO:SOIC-8_5.3x5.3mm_P1.27mm
- U10: value TPD4E05U06DQA -> TPS60403DBV; footprint Package_SON:USON-10_2.5x1.0mm_P0.5mm -> Package_TO_SOT_SMD:SOT-23-5
- U11: value SSF2215 -> LM5155DSSR; footprint Package_TO_SOT_SMD:SOT-23-6_Handsoldering -> OpenAquatix-Hardware_footprints:WSON-12-1EP_3x2mm_P0.5mm_EP1x2.65
- U13: value LM5155DSSR -> TLV75733PDRVR; footprint Package_SON:WSON-12-1EP_3x2mm_P0.5mm_EP1x2.65 -> Package_SON:WSON-6-1EP_2x2mm_P0.65mm_EP1x1.6mm
- U14: value TLV9061xDBV -> TLV75733PDRVR; footprint Package_TO_SOT_SMD:SOT-23-5 -> Package_SON:WSON-6-1EP_2x2mm_P0.65mm_EP1x1.6mm
- U15: value OPA333xxD -> LMR54406; footprint Package_SO:SOIC-8_3.9x4.9mm_P1.27mm -> Package_TO_SOT_SMD:SOT-23-6
- U16: value TLV9061xDBV -> TPD4E05U06DQA; footprint Package_TO_SOT_SMD:SOT-23-5 -> Package_SON:USON-10_2.5x1.0mm_P0.5mm
- U17: value PGA113 -> USB3343; footprint Package_SO:TSSOP-10_3x3mm_P0.5mm -> Package_DFN_QFN:QFN-24-1EP_4x4mm_P0.5mm_EP2.6x2.6mm
- U18: value TPA3132D2RHBR -> TPD4E05U06DQA; footprint Package_DFN_QFN:VQFN-32-1EP_5x5mm_P0.5mm_EP3.5x3.5mm -> Package_SON:USON-10_2.5x1.0mm_P0.5mm
- U19: value TLV9151xDBV -> OPA2316; footprint Package_TO_SOT_SMD:SOT-23-5 -> Package_SO:MSOP-10_3x3mm_P0.5mm
- U2: value TLV75733PDYDR -> STM32H723VET6; footprint Package_SON:WSON-6-1EP_2x2mm_P0.65mm_EP1x1.6mm -> Package_QFP:LQFP-100_14x14mm_P0.5mm
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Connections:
- C1 pad 1: +3V3 -> +3.3VA
- C10 pad 1: +3.3VA -> +3V3
- C100 pad 2: Net-(C100-Pad2) -> AMP_R
- C101 pad 1: Net-(C100-Pad2) -> AMP_L
- C101 pad 2: Net-(U20-+) -> GND
- C102 pad 1: +3.3VA -> GND
- C102 pad 2: GND -> Net-(C102-Pad2)
- C103 pad 1: -3V3 -> Net-(C103-Pad1)
- C104 pad 1: +3V3 -> GND
- C104 pad 2: GND -> +3V3
- C105 pad 1: GND -> Net-(U22-IN+)
- C105 pad 2: DAC_TRANSDUCER -> Net-(U22-IN-)
- C106 pad 1: +1V65 -> GND
- C106 pad 2: GND -> +3V3
- C107 pad 1: -3V3 -> Net-(C107-Pad1)
- C107 pad 2: GND -> Net-(U23-+)
- C109 pad 2: Net-(U16-+) -> GND
- C11 pad 1: /Impedance matching/TRANS_OUT -> +3V3
- C11 pad 2: TRANSDUCER_TX -> GND
- C110 pad 1: PWR_AMP_V_FB -> +3V3
- C111 pad 1: Net-(C111-Pad1) -> Net-(U24-COM)
- C111 pad 2: GND -> Net-(U25-+)
- C112 pad 1: Net-(C112-Pad1) -> +3.3VA
- C112 pad 2: Net-(U25-+) -> GND
- C113 pad 1: +3.3VA -> -3V3
- C114 pad 1: -3V3 -> +3.3VA
- C115 pad 1: GND -> -3V3
- C115 pad 2: TRANSDUCER_RX -> GND
- C12 pad 1: /Impedance matching/TRANS_OUT -> /STM32/HSE1
- C12 pad 2: TRANSDUCER_TX -> GND
- C13 pad 1: /STM32/RESET# -> ADC_IN
- C14 pad 1: /Impedance matching/TRANS_OUT -> +3V3
- C14 pad 2: TRANSDUCER_TX -> GND
- C15 pad 1: /DC-DC/5V_SW -> +3V3
- C15 pad 2: /DC-DC/5V_FB -> GND
- C16 pad 1: +BATT -> PWR_AMP_V_FB
- C17 pad 1: +BATT -> /STM32/HSE2
- C18 pad 1: /DC-DC/5V_SW -> +3V3
- C19 pad 1: /DC-DC/5V_SW -> /STM32/WS_5V
- C2 pad 1: +3V3 -> +3.3VA
- C20 pad 1: /DC-DC/5V_SW -> /STM32/USBFS_5V
- C21 pad 1: /DC-DC/5V_SW -> +BATT
- C22 pad 1: +5V -> +BATT
- C23 pad 1: +5V -> Net-(U11-SS)
- C24 pad 1: GND -> Net-(U9-VCC)
- C24 pad 2: +3V3 -> GND
- C25 pad 1: +5V -> /DC-DC/N5V_5V
- C26 pad 1: +3V3 -> /DC-DC/30V_BIAS
- C27 pad 1: +3V3 -> /DC-DC/30V_BIAS
- C28 pad 1: +3V3 -> /DC-DC/30V_COMP
- C29 pad 1: +3V3 -> /DC-DC/30V_BIAS
- C3 pad 1: +3V3 -> GND
- C3 pad 2: GND -> Net-(C3-Pad2)
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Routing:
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- added copper zone on F.Cu, net +12V
- added copper zone on In2.Cu, net +12V
- added copper zone on In2.Cu, net +3.3VA
- added copper zone on F.Cu, net +30V
- added copper zone on In2.Cu, net +30V
- added copper zone on In2.Cu, net +3V3
- added copper zone on In2.Cu, net -3V3
- added copper zone on F.Cu, net /Connections/PWR_IN1
- added copper zone on F.Cu, net /Connections/PWR_IN2
- added copper zone on F.Cu, net /DC-DC/+30Va
- added copper zone on F.Cu, net /DC-DC/30V_BIAS
- added copper zone on F.Cu, net /DC-DC/5V_SWa
- added copper zone on B.Cu, net GND
- added copper zone on In3.Cu, net GND
- removed copper zone on B.Cu, net +26V
- removed copper zone on F.Cu, net +26V
- removed copper zone on B.Cu, net +3V3
- removed copper zone on B.Cu, net +BATT
- removed copper zone on F.Cu, net /Connections/BATT_CONNa
- removed copper zone on F.Cu, net /Connections/BATT_CONNb
- removed copper zone on F.Cu, net /DC-DC/+26Va
- removed copper zone on F.Cu, net /DC-DC/Q1s
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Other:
- board size 96.2 x 96.2 mm -> 100 x 100 mm
- copper layers 4 -> 6
- board text added: "30V"
- board text added: "OpenAquatix v2.0 HW ID: 0 (0000) CERN-OHL-P-2.0 © 2025 OpenAquatix Contributors github.com/ericvoi/OpenAquatix-Hardware"
- board text added: "USB FS"
- board text added: "USB HS"
- board text removed: "*"
- board text removed: "+"
- board text removed: "+26V"
- board text removed: "-"
- board text removed: "GND"
- board text removed: "IN"
- board text removed: "USB"
